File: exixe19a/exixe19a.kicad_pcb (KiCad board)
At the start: 2 copper layers, 20 x 40 mm, 39 parts, among them J1 Conn_01x07, J2 Conn_01x07, Q1 BF820W, Q10 BF820W, Q11 BF820W, Q3 MSB92W, Q4 BF820W, Q5 BF820W, Q6 BF820W, Q7 BF820W, Q8 BF820W, Q9 BF820W, U1 STM32F042K6

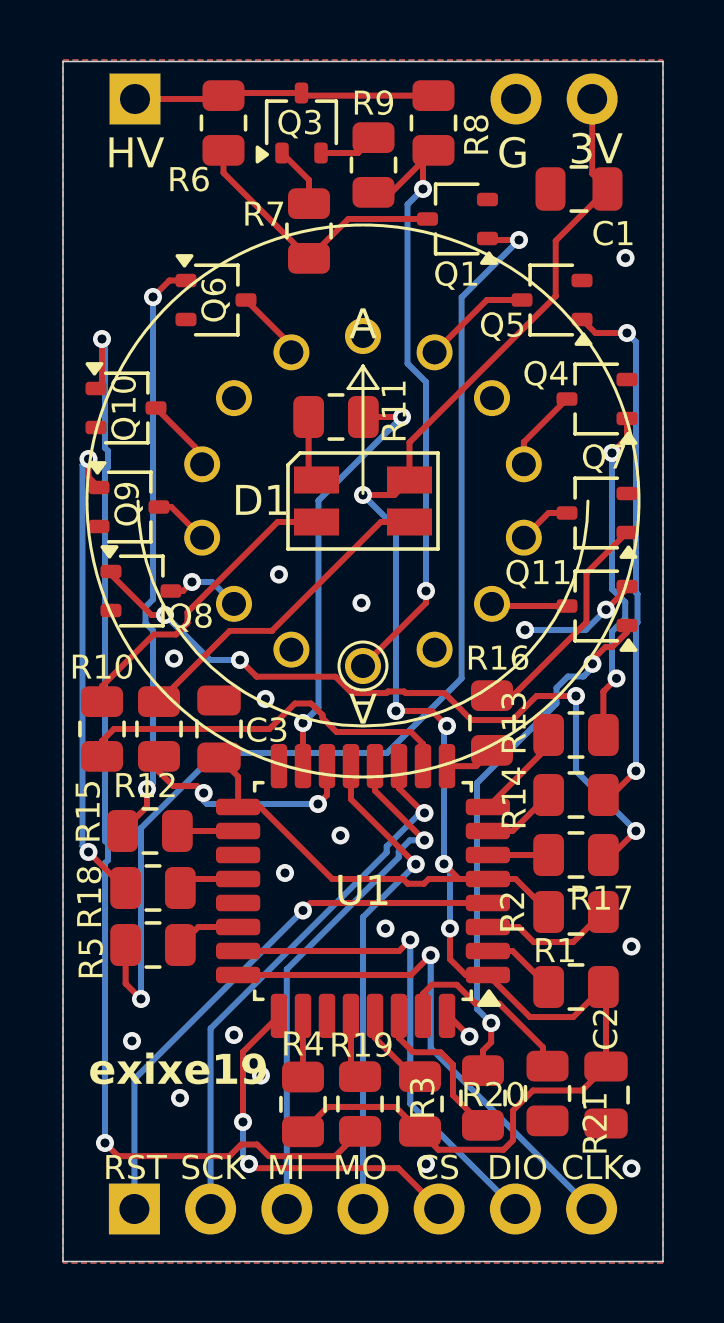
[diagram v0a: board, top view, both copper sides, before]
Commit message: new version should work
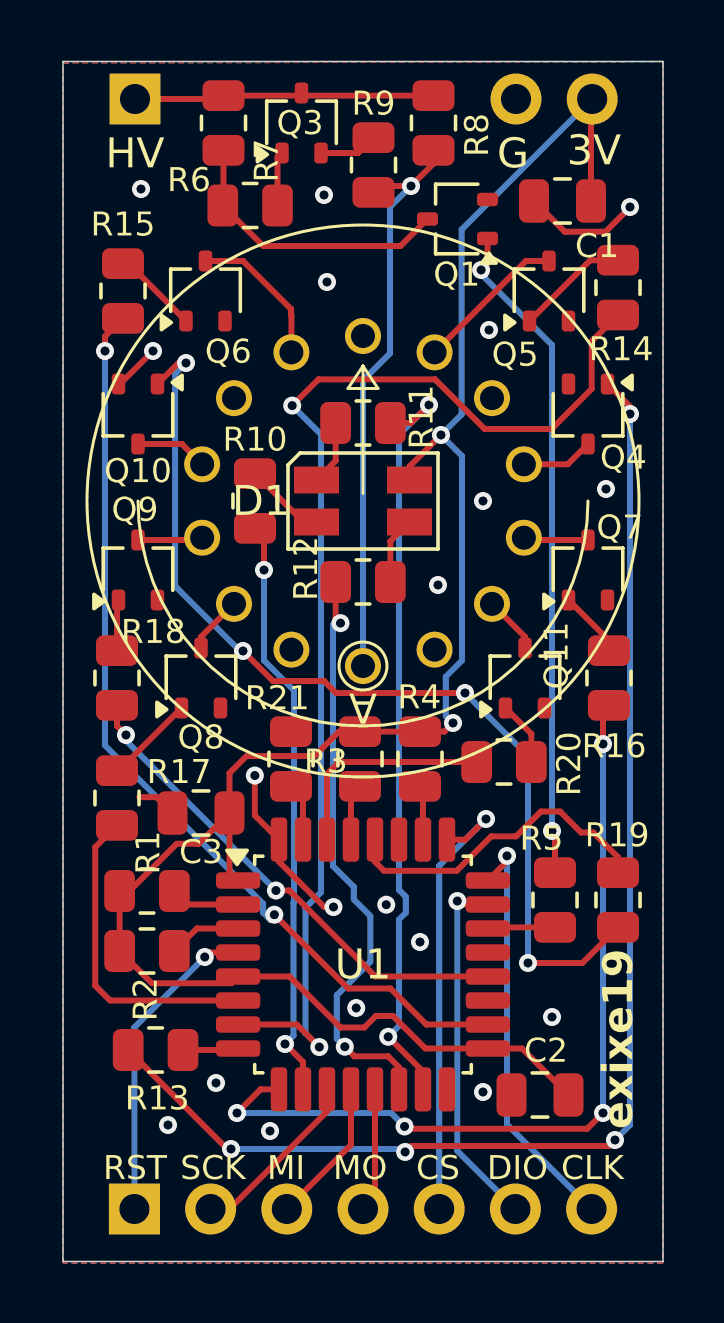
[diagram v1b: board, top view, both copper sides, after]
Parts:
- moved R15 18.0 mm to (32.0, 39.4), turned to 90 degrees
- moved R13 17.5 mm to (33.1, 64.7), turned to 180 degrees
- moved R14 17.0 mm to (48.5, 39.3), turned to 90 degrees
- moved R17 15.4 mm to (31.8, 56.3), turned to 90 degrees
- moved R1 14.7 mm to (32.8, 59.4), turned to 0 degrees
- moved R2 14.4 mm to (32.8, 61.4)
- moved R21 14.1 mm to (37.6, 55.0), turned to -90 degrees
- moved R5 13.5 mm to (46.4, 59.7), turned to 90 degrees
- moved R4 12.2 mm to (41.9, 55.0), turned to -90 degrees
- moved R3 11.7 mm to (39.9, 55.0), turned to -90 degrees
- moved R20 11.2 mm to (44.7, 55.1), turned to 0 degrees
- moved R19 11.0 mm to (48.5, 59.7)
- moved R10 9.15 mm to (36.4, 46.4)
- moved R12 8.38 mm to (40.0, 49.1), turned to 180 degrees
- moved R18 7.10 mm to (31.8, 52.3), turned to 90 degrees
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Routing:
- net /STM_1: track 2.52 -> 39.9 mm, vias 0 -> 2
- net Net-(Q4-B): track 11.4 -> 43.8 mm, vias 2 -> 4
- net /STM_8: track 2.02 -> 32.4 mm, vias 0 -> 2
- net /STM_3: track 1.72 -> 28.0 mm, vias 0 -> 4
- net Net-(Q8-B): track 24.8 -> 3.01 mm, vias 4 -> 0
- net Net-(Q6-B): track 19.8 -> 2.89 mm, vias 2 -> 0
- net Net-(Q11-B): track 17.7 -> 2.16 mm, vias 2 -> 0
- net Net-(Q1-B): track 36.9 -> 22.2 mm
- net /STM_6: track 2.05 -> 16.6 mm, vias 0 -> 2
- net Net-(Q9-B): track 16.1 -> 1.71 mm, vias 2 -> 0
- net Net-(Q5-B): track 17.9 -> 3.79 mm, vias 2 -> 0
- net /SPI_MISO: track 17.6 -> 4.87 mm, vias 1 -> 0
- net /SPI_MOSI: track 16.6 -> 4.15 mm, vias 1 -> 0
- net /SPI_SCK: track 18.2 -> 5.96 mm, vias 1 -> 0
- net /PWM_BLUE: track 7.80 -> 19.7 mm
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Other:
- board text removed: "A"
